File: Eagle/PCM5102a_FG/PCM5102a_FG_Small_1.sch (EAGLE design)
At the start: 31 parts, among them IC1 PSOC_5LP_PROTOTIYPING_KIT, IC2 PCM5102A, IC3 TA48M033F, Q1 20MHz

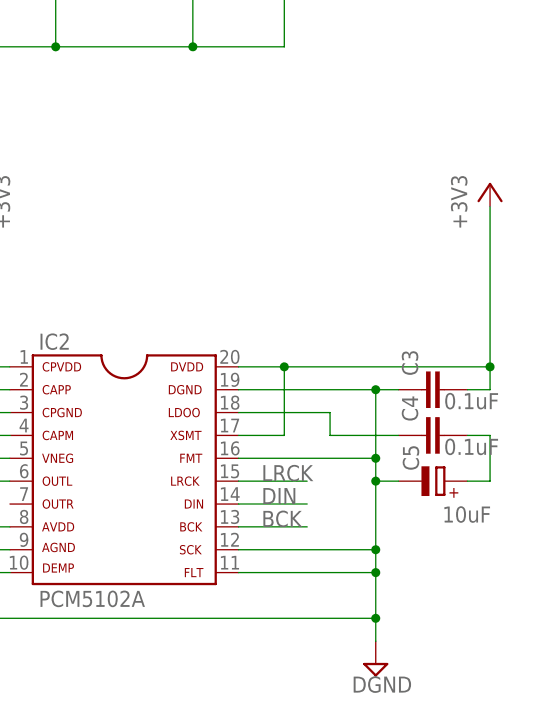
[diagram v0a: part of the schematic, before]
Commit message: ハードウェア完成
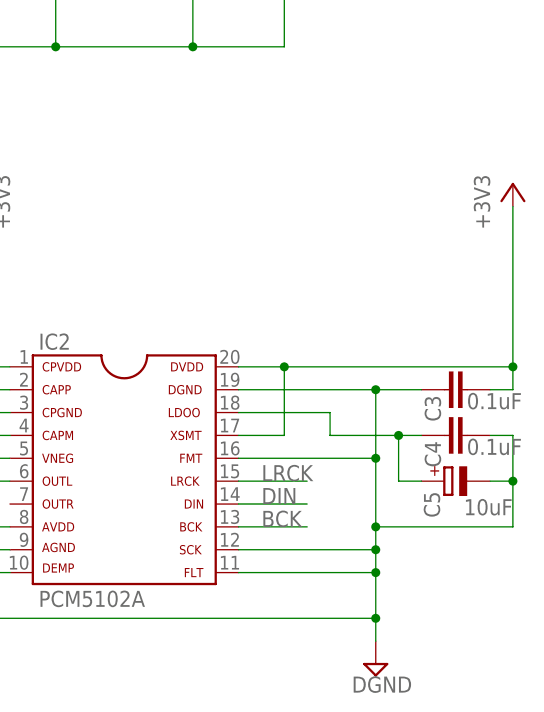
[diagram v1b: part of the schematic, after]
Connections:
- removed net N$2: C4.2, C5.+
- net DGND: now also C4.2
- net N$1: now also C5.+
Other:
- moved on the sheet: C3, C4, C5
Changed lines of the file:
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@@
 <instance part="IC2" gate="G$1" x="190.5" y="71.12"/>
 <instance part="SUPPLY4" gate="G$1" x="218.44" y="50.8"/>
-<instance part="+3V3" gate="G$1" x="231.14" y="104.14"/>
-<instance part="C3" gate="G$1" x="223.52" y="81.28" smashed="yes" rot="R90">
-<attribute name="NAME" x="223.139" y="82.804" size="1.778" layer="95" rot="R90"/>
-<attribute name="VALUE" x="232.156" y="80.899" size="1.778" layer="96" rot="R180"/>
-</instance>
-<instance part="C4" gate="G$1" x="223.52" y="76.2" smashed="yes" rot="R90">
-<attribute name="NAME" x="223.139" y="77.724" size="1.778" layer="95" rot="R90"/>
-<attribute name="VALUE" x="232.156" y="75.819" size="1.778" layer="96" rot="R180"/>
-</instance>
-<instance part="C5" gate="G$1" x="226.06" y="71.12" smashed="yes" rot="MR90">
-<attribute name="NAME" x="221.4626" y="72.263" size="1.778" layer="95" rot="MR90"/>
-<attribute name="VALUE" x="231.267" y="66.5226" size="1.778" layer="96" rot="MR0"/>
+<instance part="+3V3" gate="G$1" x="233.68" y="104.14"/>
+<instance part="C3" gate="G$1" x="226.06" y="81.28" smashed="yes" rot="R90">
+<attribute name="NAME" x="225.679" y="77.724" size="1.778" layer="95" rot="R90"/>
+<attribute name="VALUE" x="234.696" y="80.899" size="1.778" layer="96" rot="R180"/>
+</instance>
+<instance part="C4" gate="G$1" x="226.06" y="76.2" smashed="yes" rot="R90">
+<attribute name="NAME" x="225.679" y="72.644" size="1.778" layer="95" rot="R90"/>
+<attribute name="VALUE" x="234.696" y="75.819" size="1.778" layer="96" rot="R180"/>
+</instance>
+<instance part="C5" gate="G$1" x="226.06" y="71.12" smashed="yes" rot="MR270">
+<attribute name="NAME" x="225.5774" y="69.977" size="1.778" layer="95" rot="MR270"/>
+<attribute name="VALUE" x="228.219" y="69.1134" size="1.778" layer="96" rot="MR180"/>
 </instance>
 <instance part="+3V4" gate="G$1" x="172.72" y="104.14" smashed="yes">
@@
 <wire x1="218.44" y1="81.28" x2="218.44" y2="73.66" width="0.1524" layer="91"/>
 <pinref part="IC2" gate="G$1" pin="19"/>
-<wire x1="218.44" y1="73.66" x2="218.44" y2="71.12" width="0.1524" layer="91"/>
-<wire x1="218.44" y1="71.12" x2="218.44" y2="63.5" width="0.1524" layer="91"/>
+<wire x1="218.44" y1="73.66" x2="218.44" y2="66.04" width="0.1524" layer="91"/>
+<wire x1="218.44" y1="66.04" x2="218.44" y2="63.5" width="0.1524" layer="91"/>
 <wire x1="218.44" y1="63.5" x2="218.44" y2="60.96" width="0.1524" layer="91"/>
 <wire x1="218.44" y1="60.96" x2="218.44" y2="55.88" width="0.1524" layer="91"/>
@@
 <wire x1="218.44" y1="81.28" x2="203.2" y2="81.28" width="0.1524" layer="91"/>
 <pinref part="C3" gate="G$1" pin="1"/>
-<wire x1="220.98" y1="81.28" x2="218.44" y2="81.28" width="0.1524" layer="91"/>
+<wire x1="223.52" y1="81.28" x2="218.44" y2="81.28" width="0.1524" layer="91"/>
 <junction x="218.44" y="81.28"/>
 <pinref part="IC2" gate="G$1" pin="16"/>
 <wire x1="203.2" y1="73.66" x2="218.44" y2="73.66" width="0.1524" layer="91"/>
 <junction x="218.44" y="73.66"/>
-<pinref part="C5" gate="G$1" pin="-"/>
-<wire x1="220.98" y1="71.12" x2="218.44" y2="71.12" width="0.1524" layer="91"/>
-<junction x="218.44" y="71.12"/>
 <pinref part="IC2" gate="G$1" pin="11"/>
 <wire x1="203.2" y1="60.96" x2="218.44" y2="60.96" width="0.1524" layer="91"/>
@@
 <wire x1="175.26" y1="55.88" x2="218.44" y2="55.88" width="0.1524" layer="91"/>
 <junction x="218.44" y="55.88"/>
+<wire x1="218.44" y1="66.04" x2="233.68" y2="66.04" width="0.1524" layer="91"/>
+<junction x="218.44" y="66.04"/>
+<pinref part="C4" gate="G$1" pin="2"/>
+<wire x1="231.14" y1="76.2" x2="233.68" y2="76.2" width="0.1524" layer="91"/>
+<wire x1="233.68" y1="76.2" x2="233.68" y2="71.12" width="0.1524" layer="91"/>
+<pinref part="C5" gate="G$1" pin="-"/>
+<wire x1="233.68" y1="71.12" x2="233.68" y2="66.04" width="0.1524" layer="91"/>
+<wire x1="231.14" y1="71.12" x2="233.68" y2="71.12" width="0.1524" layer="91"/>
+<junction x="233.68" y="71.12"/>
 </segment>
 <segment>
@@
 <pinref part="C4" gate="G$1" pin="1"/>
 <wire x1="213.36" y1="76.2" x2="220.98" y2="76.2" width="0.1524" layer="91"/>
+<wire x1="220.98" y1="76.2" x2="223.52" y2="76.2" width="0.1524" layer="91"/>
+<wire x1="220.98" y1="76.2" x2="220.98" y2="71.12" width="0.1524" layer="91"/>
+<junction x="220.98" y="76.2"/>
+<pinref part="C5" gate="G$1" pin="+"/>
+<wire x1="223.52" y1="71.12" x2="220.98" y2="71.12" width="0.1524" layer="91"/>
 </segment>
 </net>
@@
 <pinref part="IC2" gate="G$1" pin="20"/>
 <wire x1="203.2" y1="83.82" x2="208.28" y2="83.82" width="0.1524" layer="91"/>
-<wire x1="208.28" y1="83.82" x2="231.14" y2="83.82" width="0.1524" layer="91"/>
+<wire x1="208.28" y1="83.82" x2="233.68" y2="83.82" width="0.1524" layer="91"/>
 <junction x="208.28" y="83.82"/>
 <pinref part="+3V3" gate="G$1" pin="+3V3"/>
-<wire x1="231.14" y1="83.82" x2="231.14" y2="101.6" width="0.1524" layer="91"/>
+<wire x1="233.68" y1="83.82" x2="233.68" y2="101.6" width="0.1524" layer="91"/>
 <pinref part="C3" gate="G$1" pin="2"/>
-<wire x1="228.6" y1="81.28" x2="231.14" y2="81.28" width="0.1524" layer="91"/>
-<wire x1="231.14" y1="81.28" x2="231.14" y2="83.82" width="0.1524" layer="91"/>
-<junction x="231.14" y="83.82"/>
+<wire x1="231.14" y1="81.28" x2="233.68" y2="81.28" width="0.1524" layer="91"/>
+<wire x1="233.68" y1="81.28" x2="233.68" y2="83.82" width="0.1524" layer="91"/>
+<junction x="233.68" y="83.82"/>
 </segment>
 <segment>
@@
 </segment>
 </net>
-<net name="N$2" class="0">
-<segment>
-<pinref part="C4" gate="G$1" pin="2"/>
-<wire x1="228.6" y1="76.2" x2="231.14" y2="76.2" width="0.1524" layer="91"/>
-<wire x1="231.14" y1="76.2" x2="231.14" y2="71.12" width="0.1524" layer="91"/>
-<pinref part="C5" gate="G$1" pin="+"/>
-<wire x1="231.14" y1="71.12" x2="228.6" y2="71.12" width="0.1524" layer="91"/>
-</segment>
-</net>
